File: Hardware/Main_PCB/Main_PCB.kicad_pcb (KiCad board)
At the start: 4 copper layers, 65 x 49 mm, 87 parts, among them J201 Sonar, J301 2171790001, J601 Conn_01x08_Pin, J602 Conn_01x03_Pin, J603 Servo con, SW301 TL3342F160QG_TR, SW302 TL3342F160QG_TR, U201 TUSS4470TRTJT, U301 RP2040, U302 W25Q128JVS, U401 TPS62170DSG, U402 TPS61175PWPR, U403 BD50FD0WFP2-E2, U501 ICM-42688-P, U601 NRF24L01, U602 SN74LV1T34DBV, Y301 12Mhz

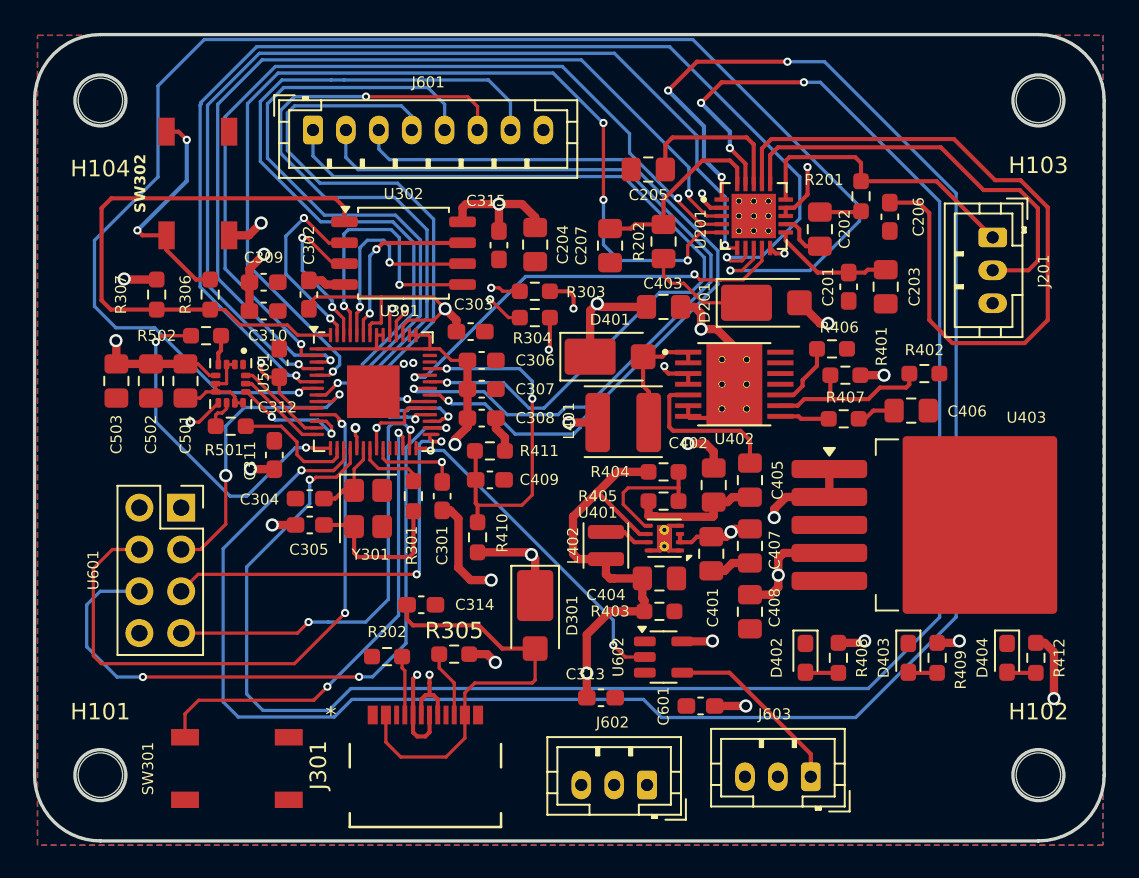
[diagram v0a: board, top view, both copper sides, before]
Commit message: V1.1 of the MainPCB
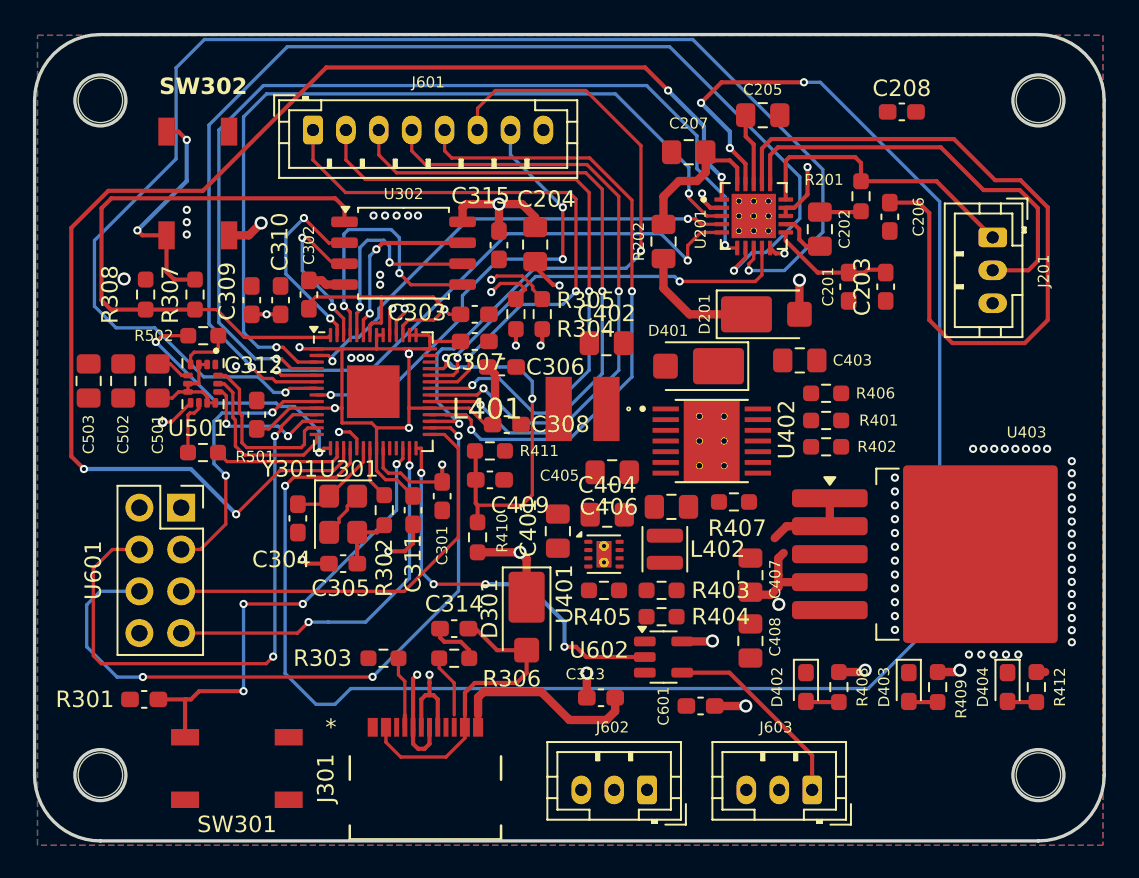
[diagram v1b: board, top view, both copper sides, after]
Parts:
- added C208: 1u, Capacitor_SMD:C_0603_1608Metric_Pad1.08x0.95mm_HandSolder, F.Cu at (116.2, 58.3)
- added R301: 10k, Capacitor_SMD:C_0603_1608Metric_Pad1.08x0.95mm_HandSolder, F.Cu at (70.2, 94.0)
- C203: value 20n -> 22n; footprint Capacitor_SMD:C_0805_2012Metric_Pad1.18x1.45mm_HandSolder -> Capacitor_SMD:C_0603_1608Metric_Pad1.08x0.95mm_HandSolder
- C206: value 2u -> 1u
- L401: footprint MainPCB:L_33uH -> MainPCB:VLCF4018
- Y301: value 12Mhz -> 12MHz
- moved C406 15.7 mm to (102.2, 82.3), turned to 180 degrees
- moved C402 10.8 mm to (98.2, 72.3), turned to 180 degrees
- moved C401 9.42 mm to (95.3, 83.8), turned to 90 degrees
- moved C311 9.07 mm to (86.5, 82.5), turned to -90 degrees
- moved C403 8.89 mm to (110.0, 73.4)
- moved R404 8.80 mm to (101.6, 89.0), turned to 0 degrees
- moved C405 8.38 mm to (98.6, 80.2), turned to 180 degrees
- moved R407 8.37 mm to (106.0, 82.0), turned to 180 degrees
- moved C205 7.70 mm to (107.8, 58.5), turned to 180 degrees
- moved R402 7.45 mm to (111.6, 78.7)
- moved C207 7.42 mm to (103.2, 60.8), turned to 180 degrees
- moved R405 6.52 mm to (98.1, 87.4)
- moved D401 5.41 mm to (103.8, 73.8), turned to 180 degrees
- moved C404 5.01 mm to (98.3, 82.8), turned to 180 degrees
- moved U401 3.80 mm to (98.1, 85.2), turned to 0 degrees
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- renumbered R301 to R302, R302 to R303, R303 to R304, R304 to R305, R305 to R306, R306 to R307, R307 to R308
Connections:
- net Net-(J301-DN1) renamed /RP2040/Data-
- net Net-(J301-DP1) renamed /RP2040/Data+
- C206 pad 1: Net-(U201-VDRV) -> GND
- C206 pad 2: GND -> Net-(U201-VDRV)
- Y301 pad 2: Net-(C305-Pad1) -> GND
- Y301 pad 3: (no net) -> Net-(C305-Pad1)
- Y301 pad 4: (no net) -> GND
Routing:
- net /OUT3: track 123.3 -> 82.9 mm
- net /RP2040/GPIO3: track 59.7 -> 35.0 mm, vias 4 -> 2
- net /RP2040/GPIO0: track 53.6 -> 29.0 mm
- net +3.3V: track 84.2 -> 65.6 mm
- net /BEMF: track 45.5 -> 28.3 mm, vias 1 -> 3
- net /AHS: track 49.8 -> 36.0 mm, vias 1 -> 2
- net GND: track 56.4 -> 43.1 mm, vias 10 -> 62
- net VDC: track 23.8 -> 10.8 mm, vias 6 -> 1
- net +12V: track 14.3 -> 2.62 mm, vias 4 -> 1
- net /ALS: track 51.0 -> 40.1 mm, vias 1 -> 2
- net Net-(U402-FB): track 10.5 -> 0.00 mm
- net Net-(U402-SS): track 9.66 -> 0.00 mm
- net /BHS: track 48.8 -> 40.0 mm, vias 1 -> 2
- net Net-(U401-FB): track 8.05 -> 0.00 mm
- net Net-(D401-A): track 7.64 -> 0.00 mm
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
